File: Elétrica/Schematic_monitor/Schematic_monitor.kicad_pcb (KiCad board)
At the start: 2 copper layers, 73.7 x 59 mm, 64 parts, among them J1 Conn_01x04, J2 USB_B_Micro, J3 Eletrode 1, J4 Eletrode 2, J5 Conn_01x09, SW1 SW_Push, SW2 SW_SPDT, U1 STM32F446RET6TR, U2 LM1117S-3.3, U3 MLX90614ESF-ACC-000-TU, U4 MAX30100EFD+, U5 AD623, U6 LM358, U7 LM358, U8 LM358, Y1 Crystal_25MHz

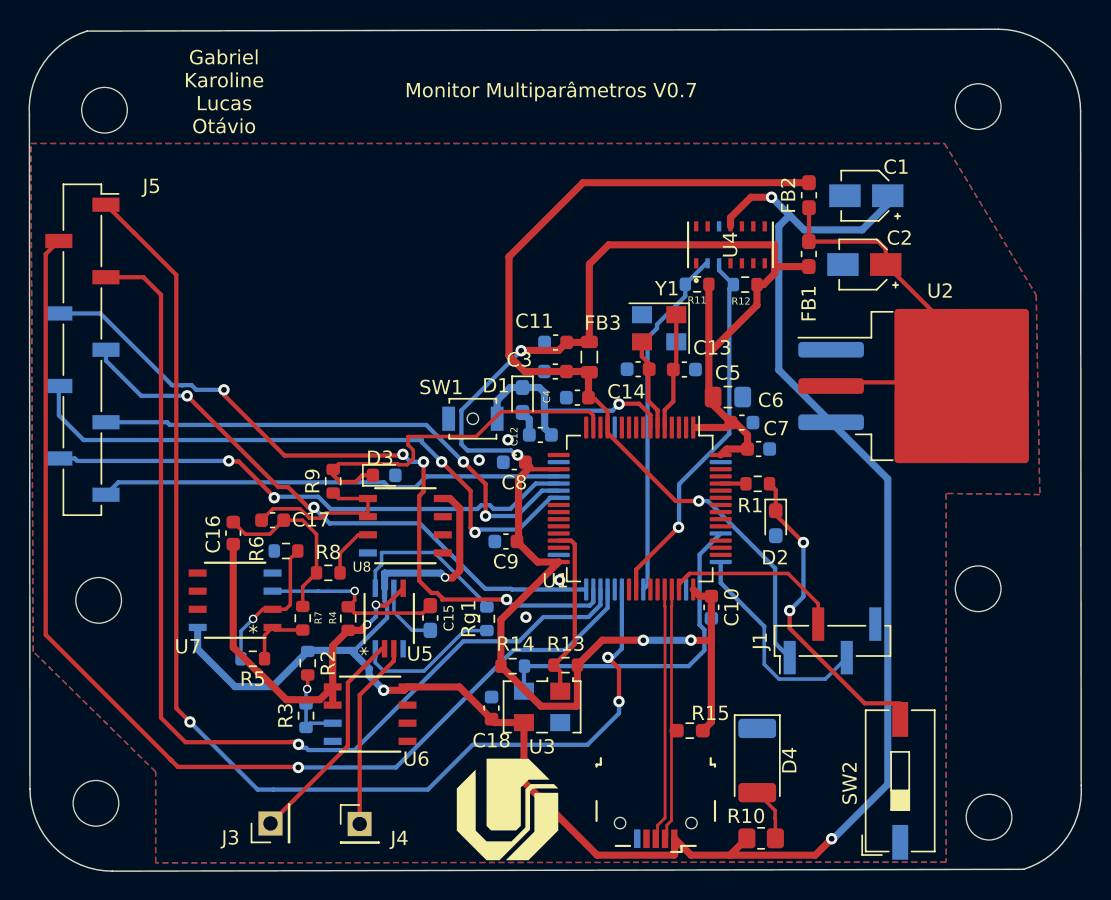
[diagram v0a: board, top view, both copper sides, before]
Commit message: PRJ4
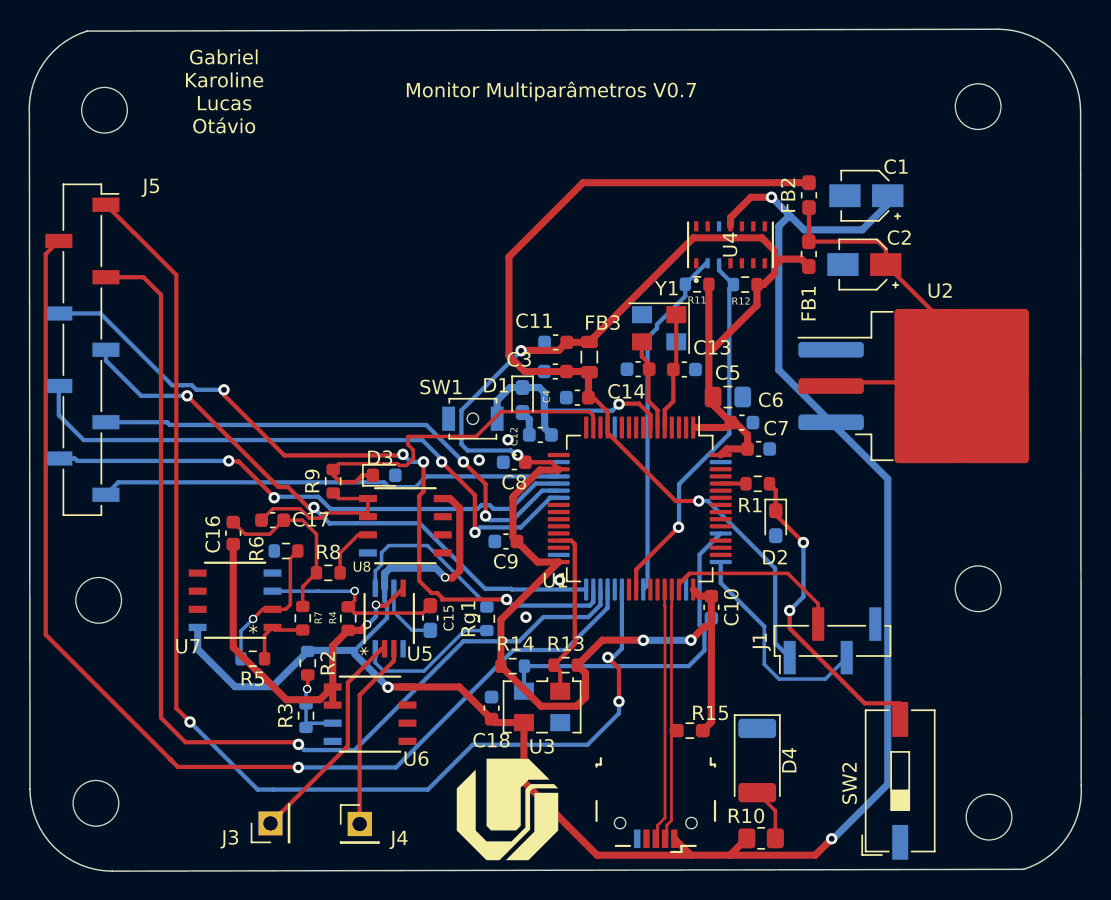
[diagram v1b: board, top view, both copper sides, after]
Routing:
- net VBUS: track 143.1 -> 142.5 mm
- net +3.3V: track 118.9 -> 118.3 mm
- removed copper zone on B.Cu, net GND
- removed copper zone on F.Cu, net GND
